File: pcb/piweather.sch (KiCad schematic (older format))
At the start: 6 parts, among them J1 Screw_Terminal_01x10, J2 Conn_01x08_Male

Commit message: wip
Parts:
- removed J1: Screw_Terminal_01x10, Main:Terminal_block_OSTVN10A150, symbol Connector:Screw_Terminal_01x10
- added J1: Screw_Terminal_01x08, Main:Terminal_block_OSTVN08A150, symbol Connector:Screw_Terminal_01x08
- added J3: Screw_Terminal_01x02, Main:TerminalBlock_1X2_P5.08mm, symbol Connector:Screw_Terminal_01x02
- added J4: Raspberry_Pi_2_3, Main:RPi_2x20_SMT, symbol Connector:Raspberry_Pi_2_3
- added U1: FT2232D, Package_QFP:LQFP-48_7x7mm_P0.5mm, symbol Interface_USB:FT2232D
- added U?: THVD1500, Main:SOIC127P490X390X175-8, symbol analog:THVD1500
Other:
- moved on the sheet: J2
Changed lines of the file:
@@
-$EndComp
-$Comp
-L Connector:Screw_Terminal_01x10 J1
-U 1 1 5D9BBCFA
-P 14500 1850
-F 0 "J1" H 14580 1842 50  0000 L CNN
-F 1 "Screw_Terminal_01x10" H 14580 1751 50  0000 L CNN
-F 2 "Main:Terminal_block_OSTVN10A150" H 14500 1850 50  0001 C CNN
-F 3 "~" H 14500 1850 50  0001 C CNN
-F 4 "On Shore Technology Inc." H 14500 1850 50  0001 C CNN "Manufacturer"
-F 5 "OSTVN10A150" H 14500 1850 50  0001 C CNN "MPN"
-	1    14500 1850
-	1    0    0    -1
 $EndComp
 $Comp
 L Connector:Conn_01x08_Male J2
 U 1 1 5D9BE108
-P 14500 3350
-F 0 "J2" H 14473 3323 50  0000 R CNN
-F 1 "Conn_01x08_Male" H 14473 3232 50  0000 R CNN
-F 2 "Main:PICOBLADE_FEMALE_8" H 14500 3350 50  0001 C CNN
-F 3 "~" H 14500 3350 50  0001 C CNN
-F 4 "Molex" H 14500 3350 50  0001 C CNN "Manufacturer"
-F 5 "0530480810" H 14500 3350 50  0001 C CNN "MPN"
-	1    14500 3350
+P 15050 3100
+F 0 "J2" H 15023 3073 50  0000 R CNN
+F 1 "Conn_01x08_Male" H 15023 2982 50  0000 R CNN
+F 2 "Main:PICOBLADE_FEMALE_8" H 15050 3100 50  0001 C CNN
+F 3 "~" H 15050 3100 50  0001 C CNN
+F 4 "Molex" H 15050 3100 50  0001 C CNN "Manufacturer"
+F 5 "0530480810" H 15050 3100 50  0001 C CNN "MPN"
+	1    15050 3100
 	-1   0    0    -1
 $EndComp
+$Comp
+L Connector:Screw_Terminal_01x02 J3
+U 1 1 5D9CB81D
+P 15050 1100
+F 0 "J3" H 15130 1092 50  0000 L CNN
+F 1 "Screw_Terminal_01x02" H 15130 1001 50  0000 L CNN
+F 2 "Main:TerminalBlock_1X2_P5.08mm" H 15050 1100 50  0001 C CNN
+F 3 "~" H 15050 1100 50  0001 C CNN
+F 4 "Phoenix Contact" H 15050 1100 50  0001 C CNN "Manufacturer"
+F 5 "1715721" H 15050 1100 50  0001 C CNN "MPN"
+	1    15050 1100
+	1    0    0    -1
+$EndComp
+$Comp
+L Connector:Screw_Terminal_01x08 J1
+U 1 1 5D9CBBE8
+P 15050 1850
+F 0 "J1" H 15130 1842 50  0000 L CNN
+F 1 "Screw_Terminal_01x08" H 15130 1751 50  0000 L CNN
+F 2 "Main:Terminal_block_OSTVN08A150" H 15050 1850 50  0001 C CNN
+F 3 "~" H 15050 1850 50  0001 C CNN
+F 4 "On Shore Technology Inc." H 15050 1850 50  0001 C CNN "Manufacturer"
+F 5 "OSTVN08A150" H 15050 1850 50  0001 C CNN "MPN"
+	1    15050 1850
+	1    0    0    -1
+$EndComp
+$Comp
+L Connector:Raspberry_Pi_2_3 J4
+U 1 1 5D9CE7F8
+P 11200 5600
+F 0 "J4" H 11200 7078 50  0000 C CNN
+F 1 "Raspberry_Pi_2_3" H 11200 6987 50  0000 C CNN
+F 2 "Main:RPi_2x20_SMT" H 11200 5600 50  0001 C CNN
+F 3 "https://www.raspberrypi.org/documentation/hardware/raspberrypi/schematics/rpi_SCH_3bplus_1p0_reduced.pdf" H 11200 5600 50  0001 C CNN
+F 4 "Harwin Inc." H 11200 5600 50  0001 C CNN "Manufacturer"
+F 5 "M20-7812045R" H 11200 5600 50  0001 C CNN "MPN"
+	1    11200 5600
+	1    0    0    -1
+$EndComp
+$Comp
+L Interface_USB:FT2232D U1
+U 1 1 5D9CF0E5
+P 4500 4900
+F 0 "U1" H 4500 6978 50  0000 C CNN
+F 1 "FT2232D" H 4500 6887 50  0000 C CNN
+F 2 "Package_QFP:LQFP-48_7x7mm_P0.5mm" H 4500 4900 50  0001 C CNN
+F 3 "http://www.ftdichip.com/Support/Documents/DataSheets/ICs/DS_FT2232D.pdf" H 4500 4900 50  0001 C CNN
+	1    4500 4900
+	1    0    0    -1
+$EndComp
+$Comp
+L analog:THVD1500 U?
+U 1 1 5D9D349A
+P 7950 5350
+F 0 "U?" H 7950 6039 60  0000 C CNN
+F 1 "THVD1500" H 7950 5933 60  0000 C CNN
+F 2 "Main:SOIC127P490X390X175-8" H 8150 4700 60  0001 C CNN
+F 3 "" H 7850 5350 60  0001 C CNN
+F 4 "Texas Instruments" H 7850 4500 60  0001 C CNN "Manufacturer"
+F 5 "THVD1500DR" H 7700 4600 60  0001 C CNN "MPN"
+	1    7950 5350
+	1    0    0    -1
+$EndComp
 $EndSCHEMATC

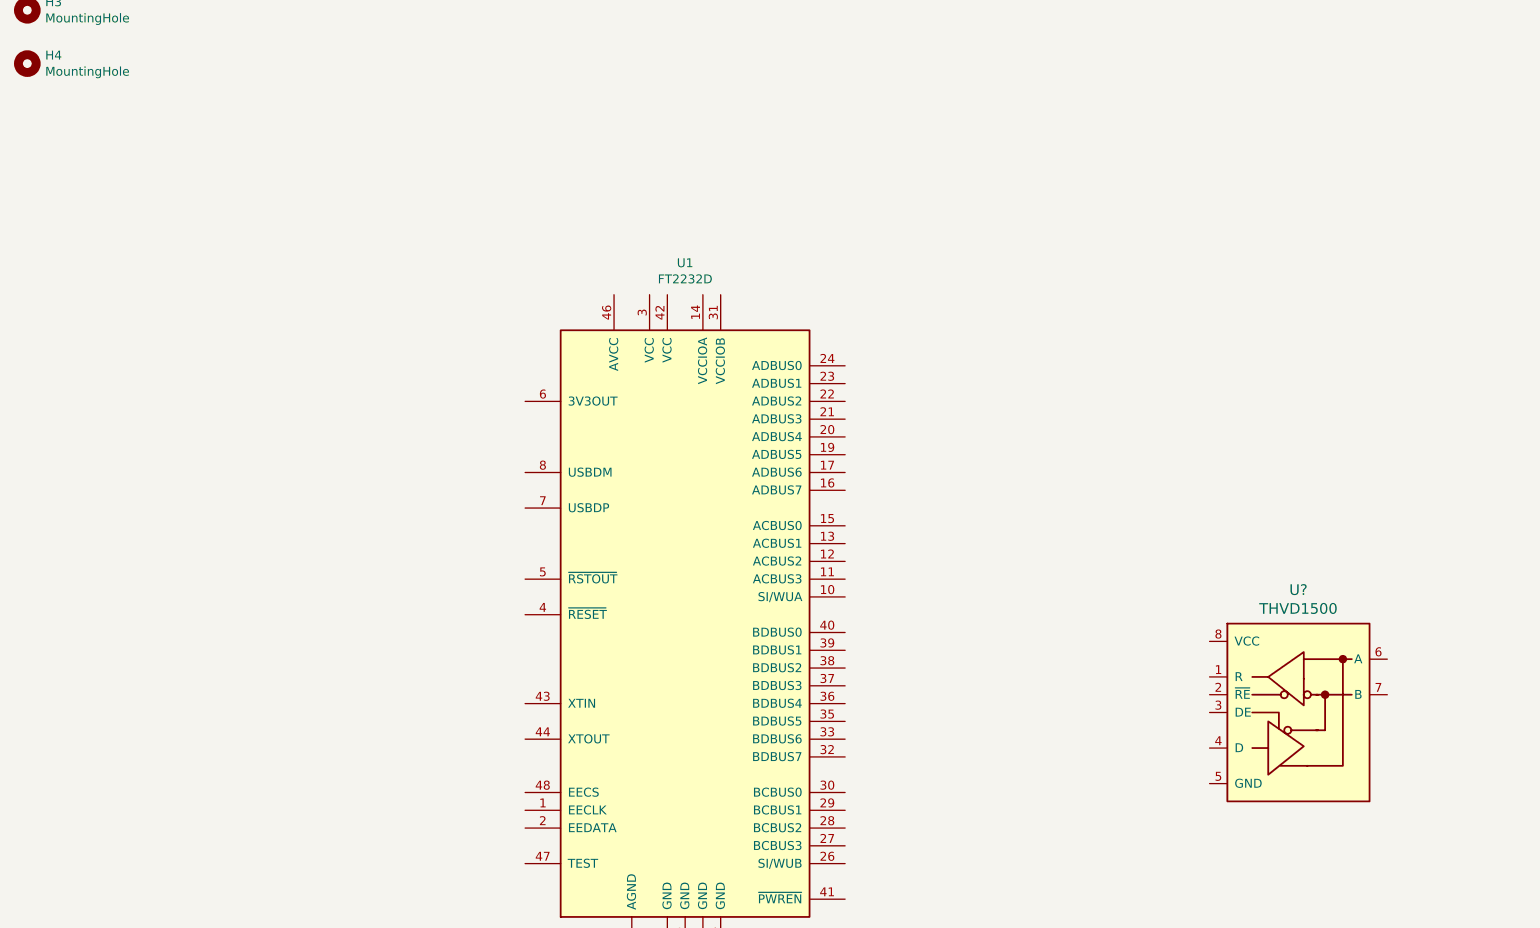
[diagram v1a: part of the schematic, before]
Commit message: wip
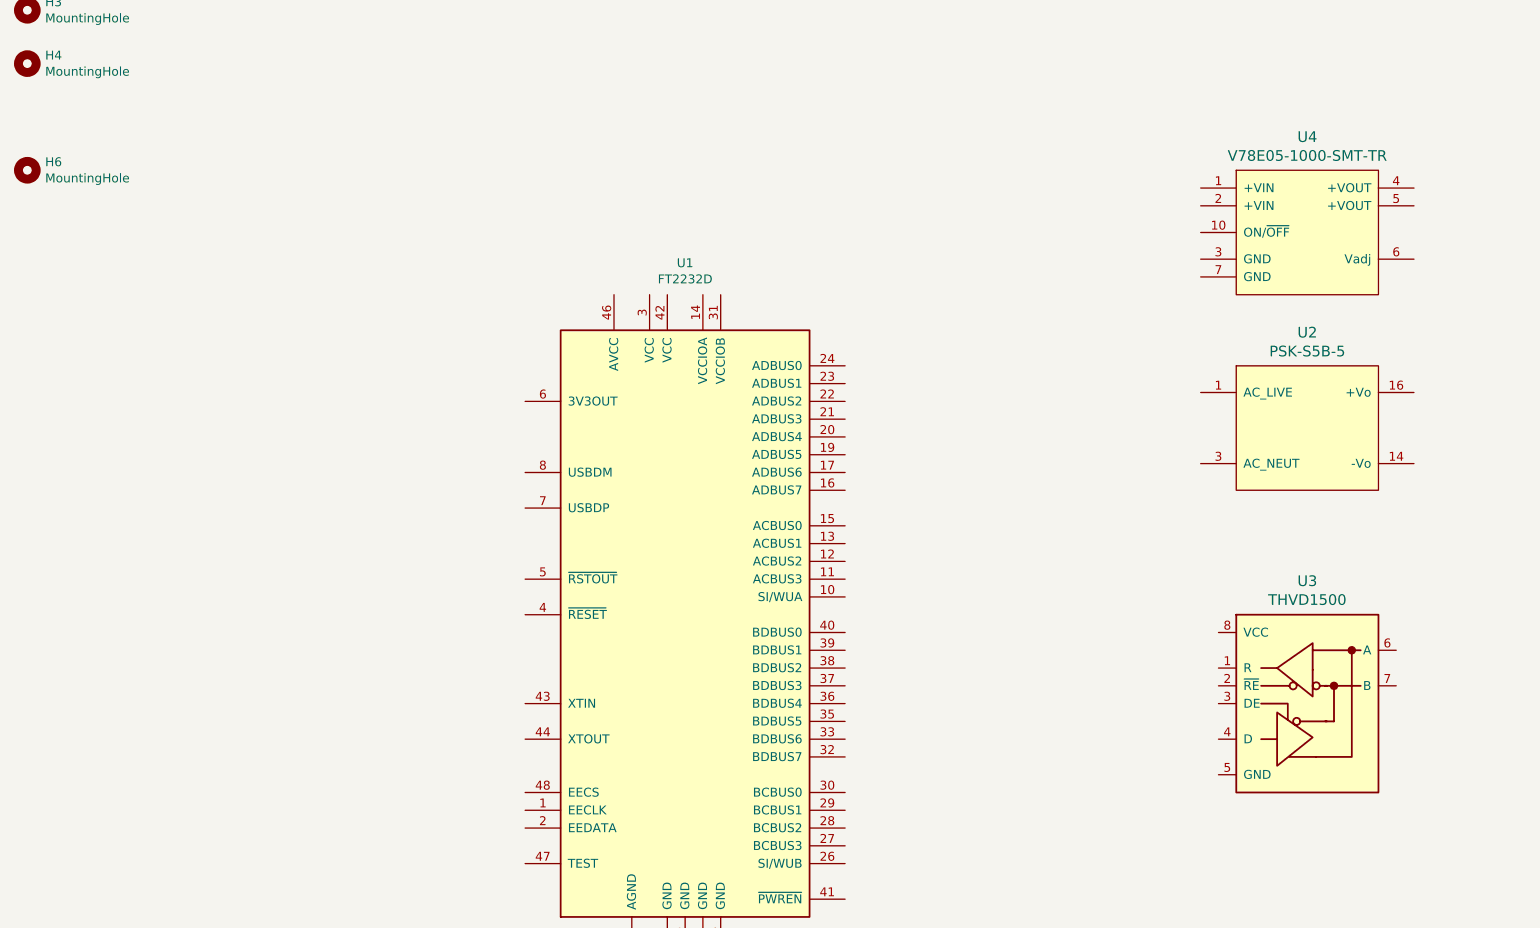
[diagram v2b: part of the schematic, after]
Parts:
- added H6: MountingHole, Main:RPi_Hat_Mounting_Hole, symbol Mechanical:MountingHole
- added U2: PSK-S5B-5, Main:PSK-S5B-5, symbol analog:PSK-S5B-5
- added U4: V78E05-1000-SMT-TR, Main:V78E05-1000-SMT-TR, symbol analog:V78E05-1000-SMT-TR
- gave numbers to parts that had none: 1
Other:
- moved on the sheet: U3
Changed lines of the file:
@@
 $EndComp
 $Comp
-L analog:THVD1500 U?
+L analog:THVD1500 U3
 U 1 1 5D9D349A
-P 7950 5350
-F 0 "U?" H 7950 6039 60  0000 C CNN
-F 1 "THVD1500" H 7950 5933 60  0000 C CNN
-F 2 "Main:SOIC127P490X390X175-8" H 8150 4700 60  0001 C CNN
-F 3 "" H 7850 5350 60  0001 C CNN
-F 4 "Texas Instruments" H 7850 4500 60  0001 C CNN "Manufacturer"
-F 5 "THVD1500DR" H 7700 4600 60  0001 C CNN "MPN"
-	1    7950 5350
+P 8000 5300
+F 0 "U3" H 8000 5989 60  0000 C CNN
+F 1 "THVD1500" H 8000 5883 60  0000 C CNN
+F 2 "Main:SOIC127P490X390X175-8" H 8200 4650 60  0001 C CNN
+F 3 "" H 7900 5300 60  0001 C CNN
+F 4 "Texas Instruments" H 7900 4450 60  0001 C CNN "Manufacturer"
+F 5 "THVD1500DR" H 7750 4550 60  0001 C CNN "MPN"
+	1    8000 5300
 	1    0    0    -1
 $EndComp
+$Comp
+L analog:PSK-S5B-5 U2
+U 1 1 5D9D3E1B
+P 8000 3750
+F 0 "U2" H 8000 4287 60  0000 C CNN
+F 1 "PSK-S5B-5" H 8000 4181 60  0000 C CNN
+F 2 "Main:PSK-S5B-5" H 7900 3150 60  0001 L CNN
+F 3 "" H 8000 3750 60  0001 C CNN
+F 4 "CUI Inc." H 7900 3250 60  0001 L CNN "Manufacturer"
+F 5 "PSK-S5B-5" H 7900 3350 60  0001 L CNN "MPN"
+	1    8000 3750
+	1    0    0    -1
+$EndComp
+$Comp
+L Mechanical:MountingHole H6
+U 1 1 5D9D426D
+P 800 2300
+F 0 "H6" H 900 2346 50  0000 L CNN
+F 1 "MountingHole" H 900 2255 50  0000 L CNN
+F 2 "Main:RPi_Hat_Mounting_Hole" H 800 2300 50  0001 C CNN
+F 3 "~" H 800 2300 50  0001 C CNN
+	1    800  2300
+	1    0    0    -1
+$EndComp
+$Comp
+L analog:V78E05-1000-SMT-TR U4
+U 1 1 5D9D532D
+P 8000 2650
+F 0 "U4" H 8000 3187 60  0000 C CNN
+F 1 "V78E05-1000-SMT-TR" H 8000 3081 60  0000 C CNN
+F 2 "Main:V78E05-1000-SMT-TR" H 7550 2100 60  0001 C CNN
+F 3 "" H 7650 2200 60  0001 C CNN
+F 4 "CUI Inc. " H 8400 2150 60  0001 L CNN "Manufacturer"
+F 5 "V78E05-1000-SMT-TR" H 8400 2250 60  0001 L CNN "MPN"
+	1    8000 2650
+	1    0    0    -1
+$EndComp

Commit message: wip
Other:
- moved on the sheet: J2
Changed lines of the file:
@@
 L Connector:Conn_01x08_Male J2
 U 1 1 5D9BE108
-P 15050 3100
-F 0 "J2" H 15023 3073 50  0000 R CNN
-F 1 "Conn_01x08_Male" H 15023 2982 50  0000 R CNN
-F 2 "Main:PICOBLADE_FEMALE_8" H 15050 3100 50  0001 C CNN
-F 3 "~" H 15050 3100 50  0001 C CNN
-F 4 "Molex" H 15050 3100 50  0001 C CNN "Manufacturer"
-F 5 "0530480810" H 15050 3100 50  0001 C CNN "MPN"
-	1    15050 3100
+P 15050 2850
+F 0 "J2" H 15023 2823 50  0000 R CNN
+F 1 "Conn_01x08_Male" H 15023 2732 50  0000 R CNN
+F 2 "Main:PICOBLADE_FEMALE_8" H 15050 2850 50  0001 C CNN
+F 3 "~" H 15050 2850 50  0001 C CNN
+F 4 "Molex" H 15050 2850 50  0001 C CNN "Manufacturer"
+F 5 "0530480810" H 15050 2850 50  0001 C CNN "MPN"
+	1    15050 2850
 	-1   0    0    -1
 $EndComp
@@
 F 5 "1715721" H 15050 1100 50  0001 C CNN "MPN"
 	1    15050 1100
-	1    0    0    -1
-$EndComp
-$Comp
-L Connector:Screw_Terminal_01x08 J1
-U 1 1 5D9CBBE8
-P 15050 1850
-F 0 "J1" H 15130 1842 50  0000 L CNN
-F 1 "Screw_Terminal_01x08" H 15130 1751 50  0000 L CNN
-F 2 "Main:Terminal_block_OSTVN08A150" H 15050 1850 50  0001 C CNN
-F 3 "~" H 15050 1850 50  0001 C CNN
-F 4 "On Shore Technology Inc." H 15050 1850 50  0001 C CNN "Manufacturer"
-F 5 "OSTVN08A150" H 15050 1850 50  0001 C CNN "MPN"
-	1    15050 1850
 	1    0    0    -1
 $EndComp
@@
 	1    0    0    -1
 $EndComp
+$Comp
+L Connector:Screw_Terminal_01x08 J1
+U 1 1 5D9E30DD
+P 15050 1800
+F 0 "J1" H 15130 1792 50  0000 L CNN
+F 1 "Screw_Terminal_01x08" H 15130 1701 50  0000 L CNN
+F 2 "Main:Terminal_block_OSTVN08A150" H 15050 1800 50  0001 C CNN
+F 3 "~" H 15050 1800 50  0001 C CNN
+F 4 "On Shore Technology Inc." H 15050 1800 50  0001 C CNN "Manufacturer"
+F 5 "OSTVN08A150" H 15050 1800 50  0001 C CNN "MPN"
+	1    15050 1800
+	1    0    0    -1
+$EndComp

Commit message: wip
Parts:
- removed J1: Screw_Terminal_01x08, Main:Terminal_block_OSTVN08A150, symbol Connector:Screw_Terminal_01x08
- removed J3: Screw_Terminal_01x02, Main:TerminalBlock_1X2_P5.08mm, symbol Connector:Screw_Terminal_01x02
- added J1: Screw_Terminal_01x10, Main:Terminal_block_OSTVN10A150, symbol Connector:Screw_Terminal_01x10
- added J3: Screw_Terminal_01x03, Main:TerminalBlock_1X3_P5.08mm, symbol Connector:Screw_Terminal_01x03
- added J? (x2): Conn_01x01_Male, symbol Connector:Conn_01x01_Male
- added U5: Si7020-A20, Package_DFN_QFN:DFN-6-1EP_3x3mm_P1mm_EP1.5x2.4mm, symbol Sensor_Humidity:Si7020-A20
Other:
- moved on the sheet: J2
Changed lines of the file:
@@
 L Connector:Conn_01x08_Male J2
 U 1 1 5D9BE108
-P 15050 2850
-F 0 "J2" H 15023 2823 50  0000 R CNN
-F 1 "Conn_01x08_Male" H 15023 2732 50  0000 R CNN
-F 2 "Main:PICOBLADE_FEMALE_8" H 15050 2850 50  0001 C CNN
-F 3 "~" H 15050 2850 50  0001 C CNN
-F 4 "Molex" H 15050 2850 50  0001 C CNN "Manufacturer"
-F 5 "0530480810" H 15050 2850 50  0001 C CNN "MPN"
-	1    15050 2850
+P 15050 3250
+F 0 "J2" H 15023 3223 50  0000 R CNN
+F 1 "Conn_01x08_Male" H 15023 3132 50  0000 R CNN
+F 2 "Main:PICOBLADE_FEMALE_8" H 15050 3250 50  0001 C CNN
+F 3 "~" H 15050 3250 50  0001 C CNN
+F 4 "Molex" H 15050 3250 50  0001 C CNN "Manufacturer"
+F 5 "0530480810" H 15050 3250 50  0001 C CNN "MPN"
+	1    15050 3250
 	-1   0    0    -1
-$EndComp
-$Comp
-L Connector:Screw_Terminal_01x02 J3
-U 1 1 5D9CB81D
-P 15050 1100
-F 0 "J3" H 15130 1092 50  0000 L CNN
-F 1 "Screw_Terminal_01x02" H 15130 1001 50  0000 L CNN
-F 2 "Main:TerminalBlock_1X2_P5.08mm" H 15050 1100 50  0001 C CNN
-F 3 "~" H 15050 1100 50  0001 C CNN
-F 4 "Phoenix Contact" H 15050 1100 50  0001 C CNN "Manufacturer"
-F 5 "1715721" H 15050 1100 50  0001 C CNN "MPN"
-	1    15050 1100
-	1    0    0    -1
 $EndComp
 $Comp
@@
 $EndComp
 $Comp
-L Connector:Screw_Terminal_01x08 J1
-U 1 1 5D9E30DD
-P 15050 1800
-F 0 "J1" H 15130 1792 50  0000 L CNN
-F 1 "Screw_Terminal_01x08" H 15130 1701 50  0000 L CNN
-F 2 "Main:Terminal_block_OSTVN08A150" H 15050 1800 50  0001 C CNN
-F 3 "~" H 15050 1800 50  0001 C CNN
-F 4 "On Shore Technology Inc." H 15050 1800 50  0001 C CNN "Manufacturer"
-F 5 "OSTVN08A150" H 15050 1800 50  0001 C CNN "MPN"
-	1    15050 1800
+L Sensor_Humidity:Si7020-A20 U5
+U 1 1 5D9E5346
+P 11000 3000
+F 0 "U5" H 11441 3046 50  0000 L CNN
+F 1 "Si7020-A20" H 11441 2955 50  0000 L CNN
+F 2 "Package_DFN_QFN:DFN-6-1EP_3x3mm_P1mm_EP1.5x2.4mm" H 11000 2600 50  0001 C CNN
+F 3 "https://www.silabs.com/documents/public/data-sheets/Si7020-A20.pdf" H 10800 3300 50  0001 C CNN
+	1    11000 3000
 	1    0    0    -1
 $EndComp
+$Comp
+L Connector:Screw_Terminal_01x03 J3
+U 1 1 5D9E5750
+P 15050 1100
+F 0 "J3" H 15130 1142 50  0000 L CNN
+F 1 "Screw_Terminal_01x03" H 15130 1051 50  0000 L CNN
+F 2 "Main:TerminalBlock_1X3_P5.08mm" H 15050 1100 50  0001 C CNN
+F 3 "~" H 15050 1100 50  0001 C CNN
+F 4 "Phoenix Contact" H 15050 1100 50  0001 C CNN "Manufacturer"
+F 5 "1715734" H 15050 1100 50  0001 C CNN "MPN"
+	1    15050 1100
+	1    0    0    -1
+$EndComp
+$Comp
+L Connector:Screw_Terminal_01x10 J1
+U 1 1 5D9E7CDE
+P 15050 1950
+F 0 "J1" H 15130 1942 50  0000 L CNN
+F 1 "Screw_Terminal_01x10" H 15130 1851 50  0000 L CNN
+F 2 "Main:Terminal_block_OSTVN10A150" H 15050 1950 50  0001 C CNN
+F 3 "~" H 15050 1950 50  0001 C CNN
+F 4 "On Shore Technology Inc." H 15050 1950 50  0001 C CNN "Manufacturer"
+F 5 "OSTVN10A150" H 15050 1950 50  0001 C CNN "MPN"
+	1    15050 1950
+	1    0    0    -1
+$EndComp
+$Comp
+L Connector:Conn_01x01_Male J?
+U 1 1 5D9E855A
+P 15050 4250
+F 0 "J?" H 15023 4273 50  0000 R CNN
+F 1 "Conn_01x01_Male" H 15023 4182 50  0000 R CNN
+F 2 "" H 15050 4250 50  0001 C CNN
+F 3 "~" H 15050 4250 50  0001 C CNN
+	1    15050 4250
+	-1   0    0    -1
+$EndComp
+$Comp
+L Connector:Conn_01x01_Male J?
+U 1 1 5D9E87D0
+P 15050 4450
+F 0 "J?" H 15023 4473 50  0000 R CNN
+F 1 "Conn_01x01_Male" H 15023 4382 50  0000 R CNN
+F 2 "" H 15050 4450 50  0001 C CNN
+F 3 "~" H 15050 4450 50  0001 C CNN
+	1    15050 4450
+	-1   0    0    -1
+$EndComp
 $EndSCHEMATC
